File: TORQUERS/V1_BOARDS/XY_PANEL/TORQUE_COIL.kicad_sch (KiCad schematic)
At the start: 41 parts, among them Q1 BSS138, Q2 BSS138, Q4 BSS138, Q5 BSS138, U1 DRV8830DGQ

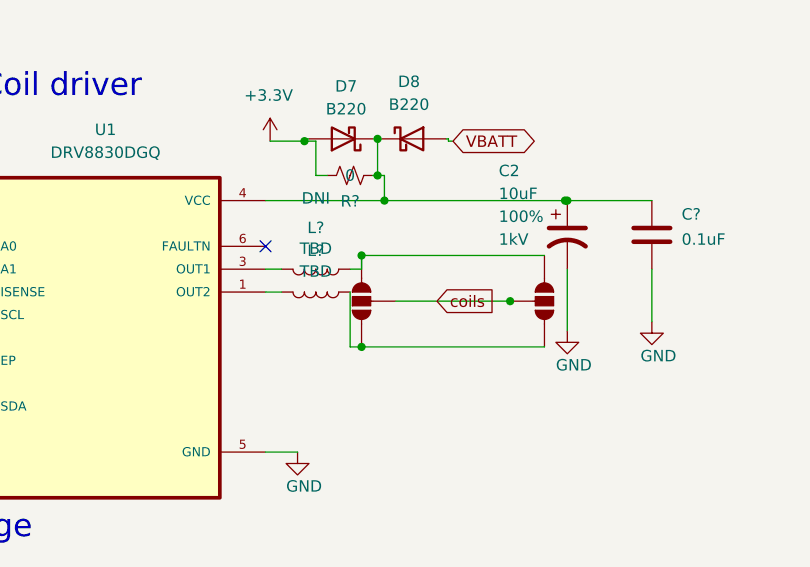
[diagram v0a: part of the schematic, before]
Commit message: made changes with feedback
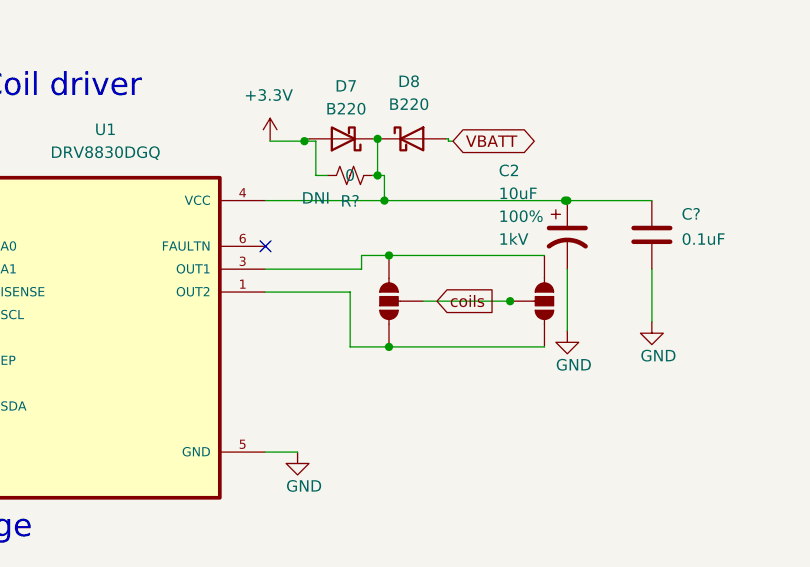
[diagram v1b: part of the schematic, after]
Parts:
- removed L? (x2): TBD, Inductor_SMD:L_0603_1608Metric, symbol Device:L
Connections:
- net at JP2.1 (A), JP2.3 (B): now also U1.1 (OUT2)
- net at JP2.1 (A), JP2.3 (B): now also U1.3 (OUT1)
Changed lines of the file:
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@@
   (junction (at 61.214 96.774) (diameter 0) (color 0 0 0 0)
   )
+  (junction (at 136.652 94.234) (diameter 0) (color 0 0 0 0)
+  )
   (junction (at 211.836 78.486) (diameter 0) (color 0 0 0 0)
   )
@@
   (junction (at 257.556 70.866) (diameter 0) (color 0 0 0 0)
   )
+  (junction (at 136.652 84.074) (diameter 0) (color 0 0 0 0)
+  )
   (junction (at 61.214 93.98) (diameter 0) (color 0 0 0 0)
   )
@@
   (junction (at 127.254 71.374) (diameter 0) (color 0 0 0 0)
   )
-  (junction (at 133.604 94.234) (diameter 0) (color 0 0 0 0)
-  )
   (junction (at 247.396 51.816) (diameter 0) (color 0 0 0 0)
   )
@@
   (junction (at 234.696 48.006) (diameter 0) (color 0 0 0 0)
   )
-  (junction (at 133.604 84.074) (diameter 0) (color 0 0 0 0)
-  )
   (junction (at 252.476 23.876) (diameter 0) (color 0 0 0 0)
   )
@@
   )
   (no_connect (at 122.936 83.058))
-  (wire (pts (xy 132.334 94.234) (xy 133.604 94.234))
-    (stroke (width 0) (type default))
-  )
   (wire (pts (xy 122.936 105.918) (xy 126.492 105.918))
     (stroke (width 0) (type default))
@@
     (stroke (width 0) (type default))
   )
-  (wire (pts (xy 122.936 85.598) (xy 124.714 85.598))
+  (wire (pts (xy 122.936 85.598) (xy 133.604 85.598))
     (stroke (width 0) (type default))
   )
@@
     (stroke (width 0) (type default))
   )
-  (wire (pts (xy 133.604 94.234) (xy 153.924 94.234))
+  (wire (pts (xy 132.334 94.234) (xy 136.652 94.234))
     (stroke (width 0) (type default))
   )
@@
     (stroke (width 0) (type default))
   )
-  (wire (pts (xy 133.604 84.074) (xy 153.924 84.074))
-    (stroke (width 0) (type default))
-  )
   (wire (pts (xy 244.856 48.006) (xy 234.696 48.006))
     (stroke (width 0) (type default))
@@
     (stroke (width 0) (type default))
   )
-  (wire (pts (xy 137.414 89.154) (xy 150.114 89.154))
+  (wire (pts (xy 140.462 89.154) (xy 150.114 89.154))
     (stroke (width 0) (type default))
   )
@@
     (stroke (width 0) (type default))
   )
-  (wire (pts (xy 122.936 88.138) (xy 124.714 88.138))
+  (wire (pts (xy 122.936 88.138) (xy 132.334 88.138))
     (stroke (width 0) (type default))
   )
@@
     (stroke (width 0) (type default))
   )
+  (wire (pts (xy 136.652 84.074) (xy 133.604 84.074))
+    (stroke (width 0) (type default))
+  )
+  (wire (pts (xy 136.652 84.074) (xy 153.924 84.074))
+    (stroke (width 0) (type default))
+  )
   (wire (pts (xy 84.074 104.14) (xy 87.376 104.14))
     (stroke (width 0) (type default))
@@
     (stroke (width 0) (type default))
   )
-  (wire (pts (xy 132.334 85.598) (xy 133.604 85.598))
-    (stroke (width 0) (type default))
-  )
   (wire (pts (xy 61.214 88.392) (xy 61.214 88.9))
     (stroke (width 0) (type default))
@@
   )
   (wire (pts (xy 135.382 71.12) (xy 135.382 75.184))
+    (stroke (width 0) (type default))
+  )
+  (wire (pts (xy 136.652 94.234) (xy 153.924 94.234))
     (stroke (width 0) (type default))
   )
@@
     )
   )
-  (symbol (lib_id "SparkFun-Jumper:SolderJumper_3_Open_No_Silk") (at 133.604 89.154 90) (unit 1)
+  (symbol (lib_id "SparkFun-Jumper:SolderJumper_3_Open_No_Silk") (at 136.652 89.154 90) (unit 1)
     (in_bom yes) (on_board yes) (dnp no) (fields_autoplaced)
-    (property "Reference" "JP2" (at 130.556 89.154 0)
-      (effects (font (size 1.27 1.27)) hide)
-    )
-    (property "Value" "~" (at 130.81 89.154 0)
+    (property "Reference" "JP2" (at 133.604 89.154 0)
+      (effects (font (size 1.27 1.27)) hide)
+    )
+    (property "Value" "~" (at 133.858 89.154 0)
       (effects (font (size 1.27 1.27)))
     )
-    (property "Footprint" "SparkFun-Jumper:SMT-JUMPER_3_NO_NO-SILK" (at 138.684 88.9 0)
-      (effects (font (size 1.27 1.27)) hide)
-    )
-    (property "Datasheet" "~" (at 139.954 89.154 0)
+    (property "Footprint" "SparkFun-Jumper:SMT-JUMPER_3_NO_NO-SILK" (at 141.732 88.9 0)
+      (effects (font (size 1.27 1.27)) hide)
+    )
+    (property "Datasheet" "~" (at 143.002 89.154 0)
       (effects (font (size 1.27 1.27)) hide)
     )
@@
         (path "/97119169-578f-44be-8822-faf8f0e4fcd6/6ee29482-1d20-4563-80a8-1ef8780df18b"
           (reference "R25") (unit 1)
-        )
-      )
-    )
-  )
-  (symbol (lib_id "Device:L") (at 128.524 85.598 270) (unit 1)
-    (in_bom yes) (on_board yes) (dnp no)
-    (property "Reference" "L?" (at 128.524 81.0006 90)
-      (effects (font (size 1.27 1.27)))
-    )
-    (property "Value" "TBD" (at 128.524 83.312 90)
-      (effects (font (size 1.27 1.27)))
-    )
-    (property "Footprint" "Inductor_SMD:L_0603_1608Metric" (at 128.524 85.598 0)
-      (effects (font (size 1.27 1.27)) hide)
-    )
-    (property "Datasheet" "~" (at 128.524 85.598 0)
-      (effects (font (size 1.27 1.27)) hide)
-    )
-    (pin "1")
-    (pin "2")
-    (instances
-      (project "xpanel"
-        (path "/30bf83b4-3f3b-46f2-ac0f-8077e2dc1b24"
-          (reference "L?") (unit 1)
-        )
-      )
-      (project "Xpanel_V1_final"
-        (path "/97119169-578f-44be-8822-faf8f0e4fcd6"
-          (reference "L1") (unit 1)
-        )
-        (path "/97119169-578f-44be-8822-faf8f0e4fcd6/db306d3f-1ab7-4e38-afab-c78bdb56c587"
-          (reference "L1") (unit 1)
-        )
-        (path "/97119169-578f-44be-8822-faf8f0e4fcd6/6ee29482-1d20-4563-80a8-1ef8780df18b"
-          (reference "L1") (unit 1)
         )
       )
@@
         )
       )
-    )
-  )
-  (symbol (lib_id "Device:L") (at 128.524 88.138 270) (unit 1)
-    (in_bom yes) (on_board yes) (dnp no)
-    (property "Reference" "L?" (at 128.524 83.5406 90)
-      (effects (font (size 1.27 1.27)))
-    )
-    (property "Value" "TBD" (at 128.524 85.852 90)
-      (effects (font (size 1.27 1.27)))
-    )
-    (property "Footprint" "Inductor_SMD:L_0603_1608Metric" (at 128.524 88.138 0)
-      (effects (font (size 1.27 1.27)) hide)
-    )
-    (property "Datasheet" "~" (at 128.524 88.138 0)
-      (effects (font (size 1.27 1.27)) hide)
-    )
-    (pin "1")
-    (pin "2")
-    (instances
-      (project "xpanel"
-        (path "/30bf83b4-3f3b-46f2-ac0f-8077e2dc1b24"
-          (reference "L?") (unit 1)
-        )
-      )
-      (project "Xpanel_V1_final"
-        (path "/97119169-578f-44be-8822-faf8f0e4fcd6"
-          (reference "L2") (unit 1)
-        )
-        (path "/97119169-578f-44be-8822-faf8f0e4fcd6/db306d3f-1ab7-4e38-afab-c78bdb56c587"
-          (reference "L2") (unit 1)
-        )
-        (path "/97119169-578f-44be-8822-faf8f0e4fcd6/6ee29482-1d20-4563-80a8-1ef8780df18b"
-          (reference "L2") (unit 1)
-        )
-      )

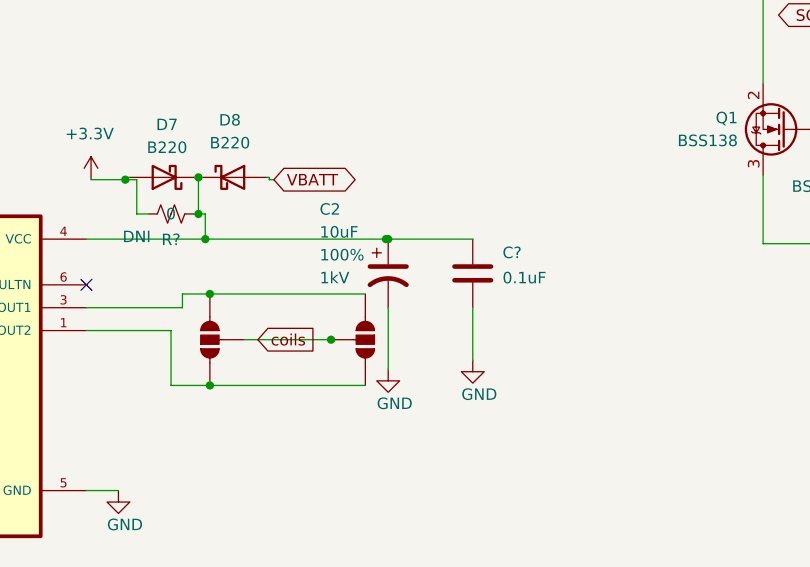
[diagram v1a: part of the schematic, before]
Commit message: made changes according to feedback
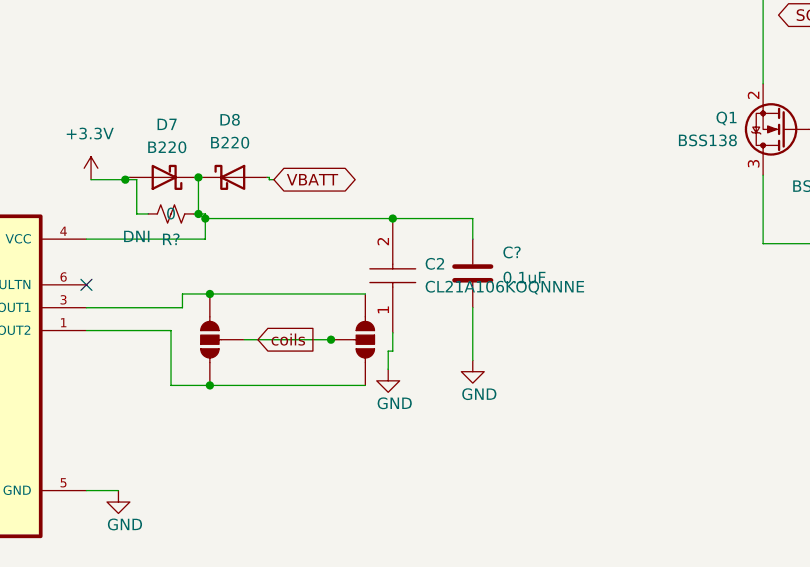
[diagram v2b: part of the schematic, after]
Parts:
- removed C2: 10uF, Capacitor_SMD:C_0805_2012Metric, symbol SparkFun-Capacitor:C_Polarized
- added C2: CL21A106KOQNNNE, CAPC2012X140N, symbol AA_AUTO_LOADER:CL21A106KOQNNNE
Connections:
- net GND: now also C2.1
- net at C?.1, D7.1 (K), D8.1 (K)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: now also C2.2
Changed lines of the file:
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@@
   (junction (at 224.536 58.166) (diameter 0) (color 0 0 0 0)
   )
+  (junction (at 136.144 75.692) (diameter 0) (color 0 0 0 0)
+  )
   (junction (at 219.456 23.876) (diameter 0) (color 0 0 0 0)
   )
-  (junction (at 156.464 77.978) (diameter 0) (color 0 0 0 0)
-  )
   (junction (at 219.456 31.496) (diameter 0) (color 0 0 0 0)
   )
@@
   (junction (at 135.382 75.184) (diameter 0) (color 0 0 0 0)
   )
-  (junction (at 156.21 77.978) (diameter 0) (color 0 0 0 0)
-  )
   (junction (at 257.556 70.866) (diameter 0) (color 0 0 0 0)
   )
@@
   (junction (at 61.214 93.98) (diameter 0) (color 0 0 0 0)
   )
+  (junction (at 156.972 75.692) (diameter 0) (color 0 0 0 0)
+  )
   (junction (at 61.214 88.9) (diameter 0) (color 0 0 0 0)
   )
@@
   )
   (junction (at 66.294 88.392) (diameter 0) (color 0 0 0 0)
-  )
-  (junction (at 136.144 77.978) (diameter 0) (color 0 0 0 0)
   )
   (junction (at 135.382 71.12) (diameter 0) (color 0 0 0 0)
@@
     (stroke (width 0) (type default))
   )
+  (wire (pts (xy 136.144 75.692) (xy 136.144 77.978))
+    (stroke (width 0) (type default))
+  )
   (wire (pts (xy 61.214 93.98) (xy 61.214 96.774))
     (stroke (width 0) (type default))
@@
     (stroke (width 0) (type default))
   )
+  (wire (pts (xy 156.464 90.424) (xy 156.464 92.456))
+    (stroke (width 0) (type default))
+  )
   (wire (pts (xy 244.856 48.006) (xy 234.696 48.006))
     (stroke (width 0) (type default))
@@
     (stroke (width 0) (type default))
   )
-  (wire (pts (xy 156.21 77.978) (xy 156.464 77.978))
-    (stroke (width 0) (type default))
-  )
   (wire (pts (xy 252.73 71.12) (xy 254 71.12))
     (stroke (width 0) (type default))
@@
     (stroke (width 0) (type default))
   )
+  (wire (pts (xy 156.972 75.692) (xy 136.144 75.692))
+    (stroke (width 0) (type default))
+  )
   (wire (pts (xy 143.256 71.374) (xy 143.764 71.374))
     (stroke (width 0) (type default))
@@
     (stroke (width 0) (type default))
   )
-  (wire (pts (xy 156.21 78.232) (xy 156.464 78.232))
-    (stroke (width 0) (type default))
-  )
   (wire (pts (xy 213.106 53.086) (xy 214.376 53.086))
     (stroke (width 0) (type default))
@@
     (stroke (width 0) (type default))
   )
+  (wire (pts (xy 156.972 88.392) (xy 156.972 90.424))
+    (stroke (width 0) (type default))
+  )
   (wire (pts (xy 143.002 71.12) (xy 143.256 71.12))
     (stroke (width 0) (type default))
@@
     (stroke (width 0) (type default))
   )
-  (wire (pts (xy 136.144 75.184) (xy 136.144 77.978))
+  (wire (pts (xy 136.144 75.184) (xy 136.144 75.692))
     (stroke (width 0) (type default))
   )
@@
     (stroke (width 0) (type default))
   )
+  (wire (pts (xy 156.972 90.424) (xy 156.464 90.424))
+    (stroke (width 0) (type default))
+  )
   (wire (pts (xy 66.294 88.138) (xy 87.376 88.138))
     (stroke (width 0) (type default))
@@
     (stroke (width 0) (type default))
   )
-  (wire (pts (xy 156.464 85.598) (xy 156.464 92.456))
-    (stroke (width 0) (type default))
-  )
   (wire (pts (xy 135.382 71.12) (xy 135.382 75.184))
     (stroke (width 0) (type default))
@@
     (stroke (width 0) (type default))
   )
-  (wire (pts (xy 156.21 78.232) (xy 156.21 77.978))
-    (stroke (width 0) (type default))
-  )
-  (wire (pts (xy 156.464 77.978) (xy 165.862 77.978))
-    (stroke (width 0) (type default))
-  )
   (wire (pts (xy 61.976 82.55) (xy 63.754 82.55))
     (stroke (width 0) (type default))
@@
     (stroke (width 0) (type default))
   )
+  (wire (pts (xy 165.862 75.692) (xy 156.972 75.692))
+    (stroke (width 0) (type default))
+  )
   (wire (pts (xy 252.476 50.546) (xy 252.476 48.006))
     (stroke (width 0) (type default))
@@
     (stroke (width 0) (type default))
   )
+  (wire (pts (xy 165.862 77.978) (xy 165.862 75.692))
+    (stroke (width 0) (type default))
+  )
   (wire (pts (xy 257.556 63.246) (xy 257.556 58.166))
     (stroke (width 0) (type default))
@@
   )
   (wire (pts (xy 127.762 71.12) (xy 127.254 71.12))
-    (stroke (width 0) (type default))
-  )
-  (wire (pts (xy 136.144 77.978) (xy 156.21 77.978))
     (stroke (width 0) (type default))
   )
@@
         (path "/97119169-578f-44be-8822-faf8f0e4fcd6/6ee29482-1d20-4563-80a8-1ef8780df18b"
           (reference "#PWR013") (unit 1)
-        )
-      )
-    )
-  )
-  (symbol (lib_id "SparkFun-Capacitor:C_Polarized") (at 156.464 81.788 0) (unit 1)
-    (in_bom yes) (on_board yes) (dnp no)
-    (property "Reference" "C2" (at 148.844 74.676 0)
-      (effects (font (size 1.27 1.27)) (justify left))
-    )
-    (property "Value" "10uF" (at 148.844 77.216 0)
-      (effects (font (size 1.27 1.27)) (justify left))
-    )
-    (property "Footprint" "Capacitor_SMD:C_0805_2012Metric" (at 156.464 81.788 0)
-      (effects (font (size 1.27 1.27)) hide)
-    )
-    (property "Datasheet" "[link text](https://cdn.sparkfun.com/assets/8/a/4/a/5/Kemet_Capacitor_Datasheet.pdf)" (at 157.734 97.028 0)
-      (effects (font (size 1.27 1.27)) hide)
-    )
-    (property "PROD_ID" "CAP-00000" (at 156.464 94.488 0)
-      (effects (font (size 1.27 1.27)) hide)
-    )
-    (property "Tolerance" "100%" (at 148.844 79.756 0)
-      (effects (font (size 1.27 1.27)) (justify left))
-    )
-    (property "Voltage" "1kV" (at 148.844 82.296 0)
-      (effects (font (size 1.27 1.27)) (justify left))
-    )
-    (pin "1")
-    (pin "2")
-    (instances
-      (project "Xpanel_V1_final"
-        (path "/97119169-578f-44be-8822-faf8f0e4fcd6"
-          (reference "C2") (unit 1)
-        )
-        (path "/97119169-578f-44be-8822-faf8f0e4fcd6/db306d3f-1ab7-4e38-afab-c78bdb56c587"
-          (reference "C6") (unit 1)
-        )
-        (path "/97119169-578f-44be-8822-faf8f0e4fcd6/6ee29482-1d20-4563-80a8-1ef8780df18b"
-          (reference "C6") (unit 1)
         )
       )
@@
         )
       )
+    )
+  )
+  (symbol (lib_id "AA_AUTO_LOADER:CL21A106KOQNNNE") (at 156.972 88.392 90) (unit 1)
+    (in_bom yes) (on_board yes) (dnp no) (fields_autoplaced)
+    (property "Reference" "C2" (at 160.528 80.772 90)
+      (effects (font (size 1.27 1.27)) (justify right))
+    )
+    (property "Value" "CL21A106KOQNNNE" (at 160.528 83.312 90)
+      (effects (font (size 1.27 1.27)) (justify right))
+    )
+    (property "Footprint" "CAPC2012X140N" (at 155.702 79.502 0)
+      (effects (font (size 1.27 1.27)) (justify left) hide)
+    )
+    (property "Datasheet" "https://datasheet.datasheetarchive.com/originals/distributors/Datasheets_SAMA/0289c6d4f30f89b64e7dd5b6a9ee99f0.pdf" (at 158.242 79.502 0)
+      (effects (font (size 1.27 1.27)) (justify left) hide)
+    )
+    (property "Description" "Samsung Electro-Mechanics 0805 (2012M) 10uF MLCC 16V dc +/-10% SMD CL21A106KOQNNNE" (at 160.782 79.502 0)
+      (effects (font (size 1.27 1.27)) (justify left) hide)
+    )
+    (property "Height" "1.4" (at 163.322 79.502 0)
+      (effects (font (size 1.27 1.27)) (justify left) hide)
+    )
+    (property "Manufacturer_Name" "SAMSUNG" (at 165.862 79.502 0)
+      (effects (font (size 1.27 1.27)) (justify left) hide)
+    )
+    (property "Manufacturer_Part_Number" "CL21A106KOQNNNE" (at 168.402 79.502 0)
+      (effects (font (size 1.27 1.27)) (justify left) hide)
+    )
+    (property "Mouser Part Number" "187-CL21A106KOQNNNE" (at 170.942 79.502 0)
+      (effects (font (size 1.27 1.27)) (justify left) hide)
+    )
+    (property "Mouser Price/Stock" "https://www.mouser.co.uk/ProductDetail/Samsung-Electro-Mechanics/CL21A106KOQNNNE?qs=349EhDEZ59qKIX0T0PKtPw%3D%3D" (at 173.482 79.502 0)
+      (effects (font (size 1.27 1.27)) (justify left) hide)
+    )
+    (property "Arrow Part Number" "CL21A106KOQNNNE" (at 176.022 79.502 0)
+      (effects (font (size 1.27 1.27)) (justify left) hide)
+    )
+    (property "Arrow Price/Stock" "https://www.arrow.com/en/products/cl21a106koqnnne/samsung-electro-mechanics?region=nac" (at 178.562 79.502 0)
+      (effects (font (size 1.27 1.27)) (justify left) hide)
+    )
+    (pin "1")
+    (pin "2")
+    (instances
+      (project "Xpanel_V1_final"
+        (path "/97119169-578f-44be-8822-faf8f0e4fcd6/6ee29482-1d20-4563-80a8-1ef8780df18b"
+          (reference "C2") (unit 1)
+        )
+      )
